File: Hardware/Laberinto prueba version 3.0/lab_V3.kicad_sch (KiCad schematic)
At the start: 27 parts, among them J1 MotorIzq, J10 DRV8833_IN, J11 DRV8833_OUT, J2 MotorDer, J3 SWITCH, J4 Jack_Batt, J5 Distancia_Izq, J6 Distancia_Frontal, J7 Distancia_Der, J8 Encoder_DER, J9 Encoder_IZQ, SW1 SW_Push, SW2 SW_Push, U1 L7805, U2 QRE1113, U3 ESP32_DevKit_V1_CH9102X

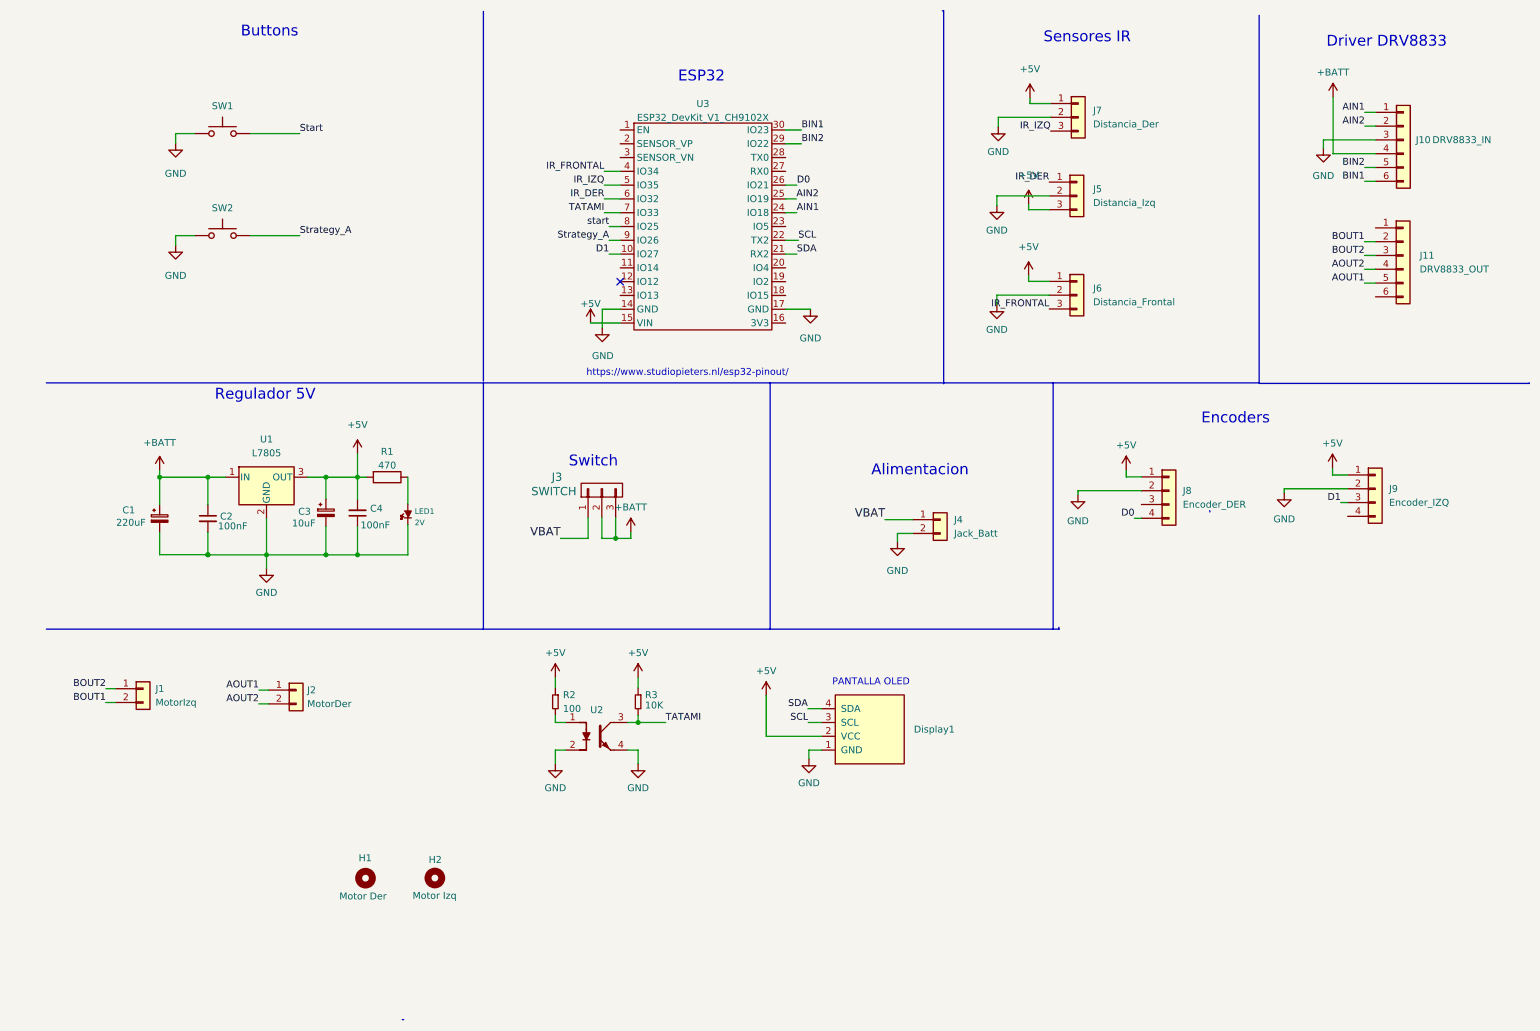
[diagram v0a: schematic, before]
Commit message: continuamos PCB
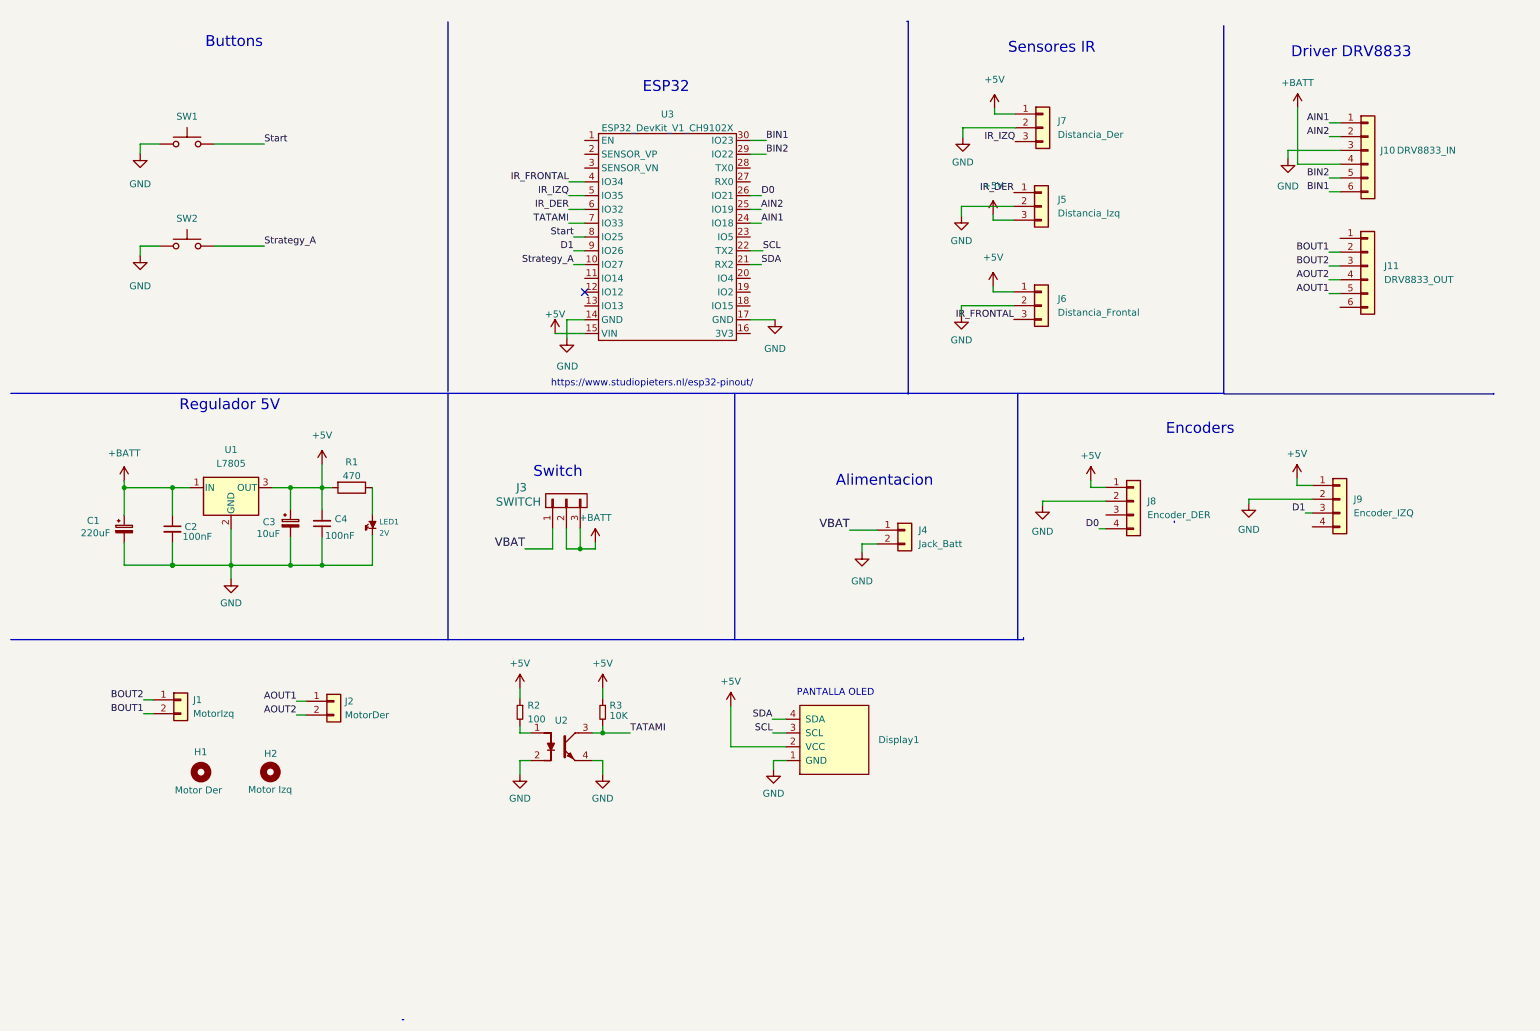
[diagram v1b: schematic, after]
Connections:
- net start is gone; now on net Start: U3.8 (IO25)
- net D1: now also U3.9 (IO26); no longer U3.10 (IO27)
- net Strategy_A: now also U3.10 (IO27); no longer U3.9 (IO26)
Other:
- moved on the sheet: C1, C2, C3, C4, Display1, H1, H2, J1, J10, J11, J2, J3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
